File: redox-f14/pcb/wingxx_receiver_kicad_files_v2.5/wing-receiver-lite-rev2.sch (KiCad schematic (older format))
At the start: 27 parts, among them IC2 XC6206P332MR, U1 ATmega32U4-AU, X1 Crystal_GND24

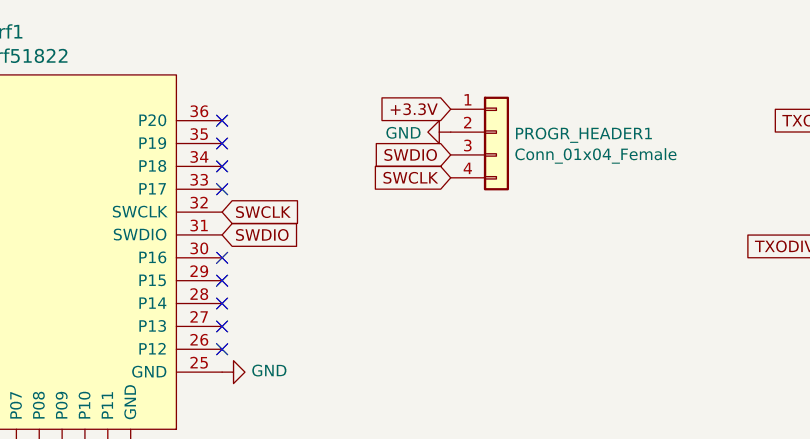
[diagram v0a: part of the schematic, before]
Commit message: new receiver
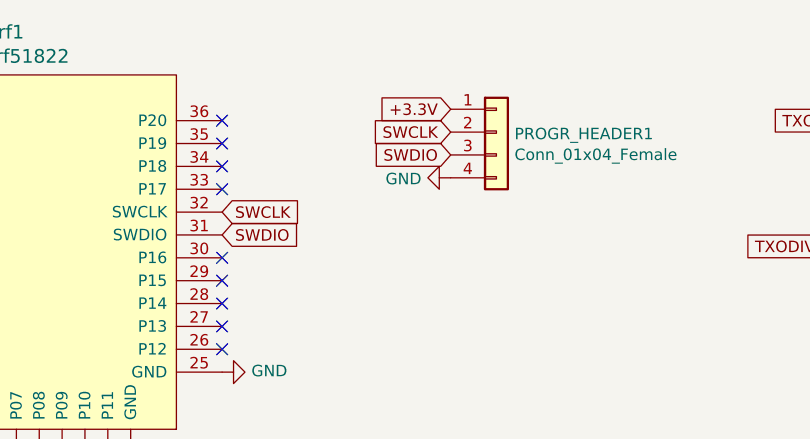
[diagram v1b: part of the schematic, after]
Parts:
- IC2: footprint SOT95P280X130-3N -> XC6206P332MR:SOT95P280X130-3N
- USB1: footprint Type-C:HRO-TYPE-C-31-M-12-HandSoldering -> pcb:HRO-TYPE-C-f14
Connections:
- net GND: now also PROGR_HEADER1.4 (Pin_4); no longer PROGR_HEADER1.2 (Pin_2)
- net SWCLK: now also PROGR_HEADER1.2 (Pin_2); no longer PROGR_HEADER1.4 (Pin_4)
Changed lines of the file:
@@
 EESchema Schematic File Version 4
+LIBS:wing-receiver-lite-rev2-cache
 EELAYER 29 0
 EELAYER END
@@
 L wingxx-receiver-v4-rescue:GND-power-redox-receiver-rescue #PWR0105
 U 1 1 5C0D4CCC
-P 3900 1100
-F 0 "#PWR0105" H 3900 850 50  0001 C CNN
-F 1 "GND" V 3905 972 50  0000 R CNN
-F 2 "" H 3900 1100 50  0001 C CNN
-F 3 "" H 3900 1100 50  0001 C CNN
-	1    3900 1100
-	0    1    1    0
-$EndComp
-Text GLabel 3900 1300 0    50   Input ~ 0
+P 3900 1300
+F 0 "#PWR0105" H 3900 1050 50  0001 C CNN
+F 1 "GND" V 3905 1172 50  0000 R CNN
+F 2 "" H 3900 1300 50  0001 C CNN
+F 3 "" H 3900 1300 50  0001 C CNN
+	1    3900 1300
+	0    1    1    0
+$EndComp
+Text GLabel 3900 1100 0    50   Input ~ 0
 SWCLK
 Text GLabel 3900 1200 0    50   Input ~ 0
@@
 F 0 "USB1" H 6183 5797 60  0000 C CNN
 F 1 "HRO-TYPE-C-31-M-12" H 6183 5691 60  0000 C CNN
-F 2 "Type-C:HRO-TYPE-C-31-M-12-HandSoldering" H 6350 5000 60  0001 C CNN
+F 2 "pcb:HRO-TYPE-C-f14" H 6350 5000 60  0001 C CNN
 F 3 "" H 6350 5000 60  0001 C CNN
 	1    6350 5000
@@
 F 0 "IC2" H 9300 1565 50  0000 C CNN
 F 1 "XC6206P332MR" H 9300 1474 50  0000 C CNN
-F 2 "SOT95P280X130-3N" H 9700 1400 50  0001 L CNN
+F 2 "XC6206P332MR:SOT95P280X130-3N" H 9700 1400 50  0001 L CNN
 F 3 "http://www.torexsemi.com/products/voltage_regulators/data/XC6206.pdf" H 9700 1300 50  0001 L CNN
 F 4 "Low ESR Cap.Compatible Postive Voltage Regulators" H 9700 1200 50  0001 L CNN "Description"
